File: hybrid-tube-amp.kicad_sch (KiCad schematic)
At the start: 11 parts, among them J101 282834-2, J102 282834-2, J103 1711725, J104 1711725, K101 RT424012F

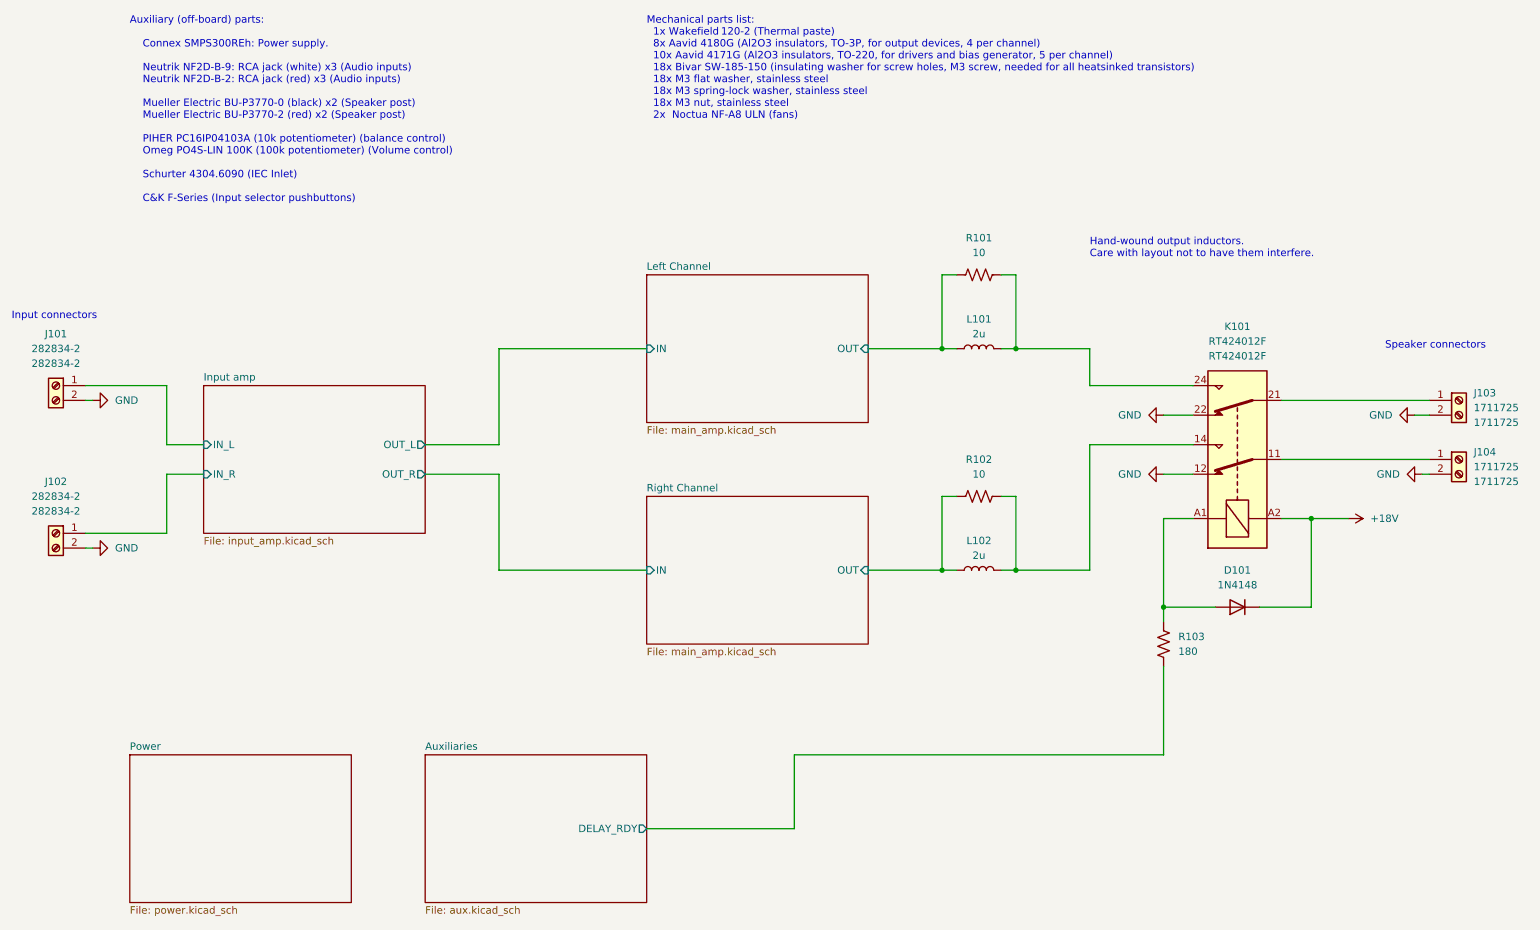
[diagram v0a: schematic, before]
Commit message: Completed schematic
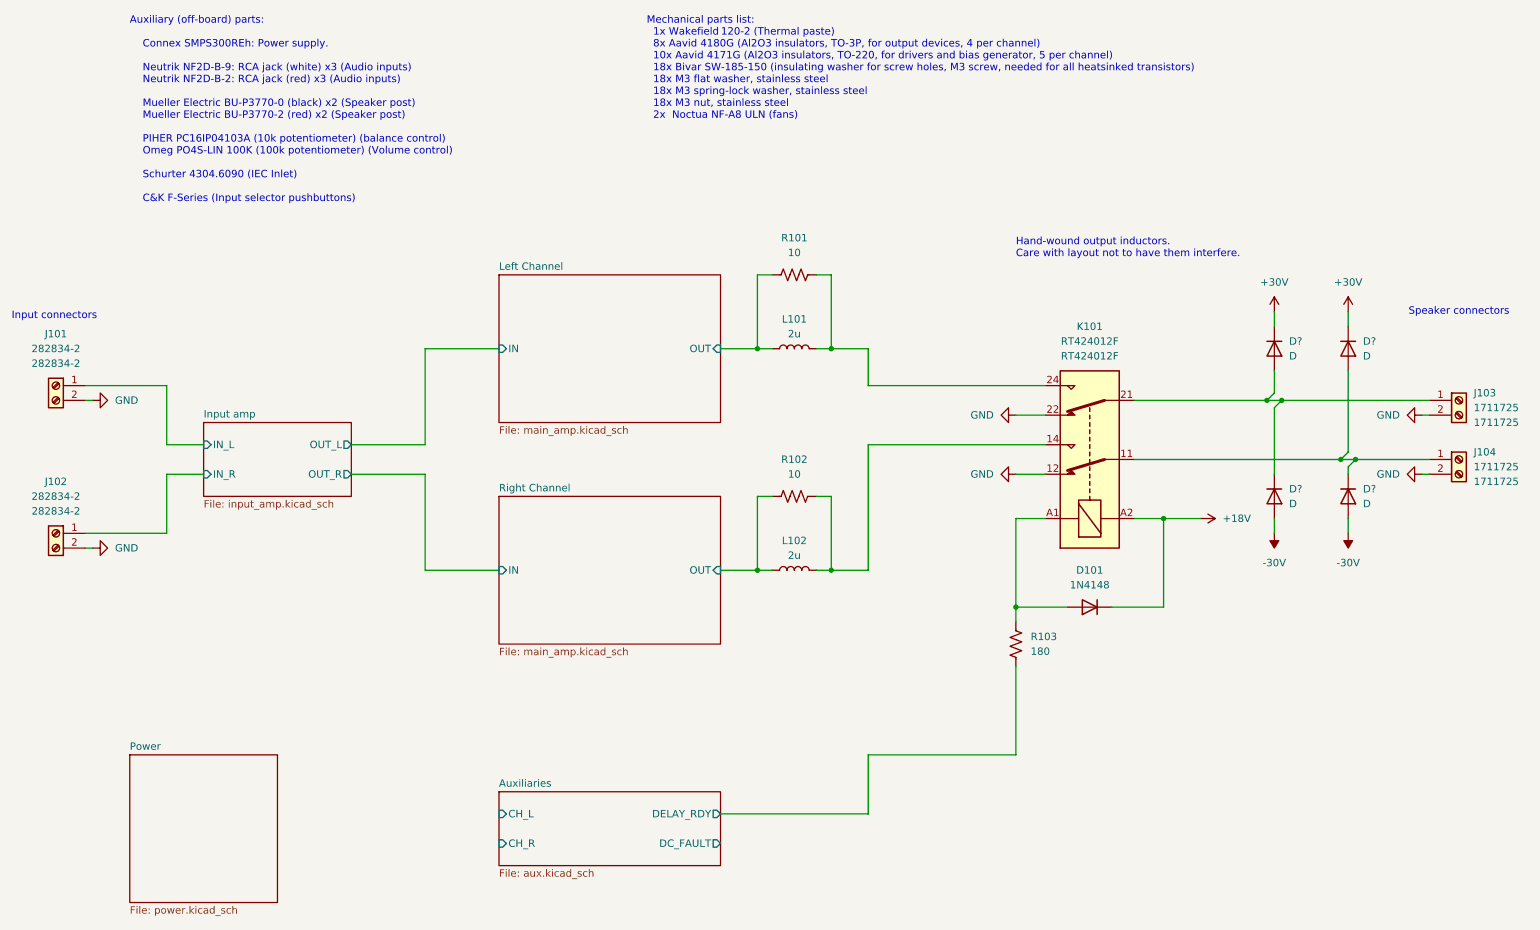
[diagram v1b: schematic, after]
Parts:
- added D? (x4): D, symbol Device:D
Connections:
- net at J104.1 (Pin_1), K101.11: now also D?.1 (K), D?.2 (A)
- net at J103.1 (Pin_1), K101.21: now also D?.1 (K), D?.2 (A)
- new net +30V: D?.1 (K), D?.1 (K)
- new net -30V: D?.2 (A), D?.2 (A)
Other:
- sheet Auxiliaries ports: added CH_L, CH_R, DC_FAULT; removed none
- moved on the sheet: D101, K101, L101, L102, R101, R102, R103
